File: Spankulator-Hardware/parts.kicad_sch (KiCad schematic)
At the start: 53 parts, among them J10 FRAM Pins, J11 OLED Pins, J14 Eurorack Power Cable, M1 FRAM_Module, M2 OLED, U10 CD4013BE split, U11 TL072CP full, U12 TL072CP full, U7 TL072CP split, U8 TL072CP split, U9 MAX7480 split

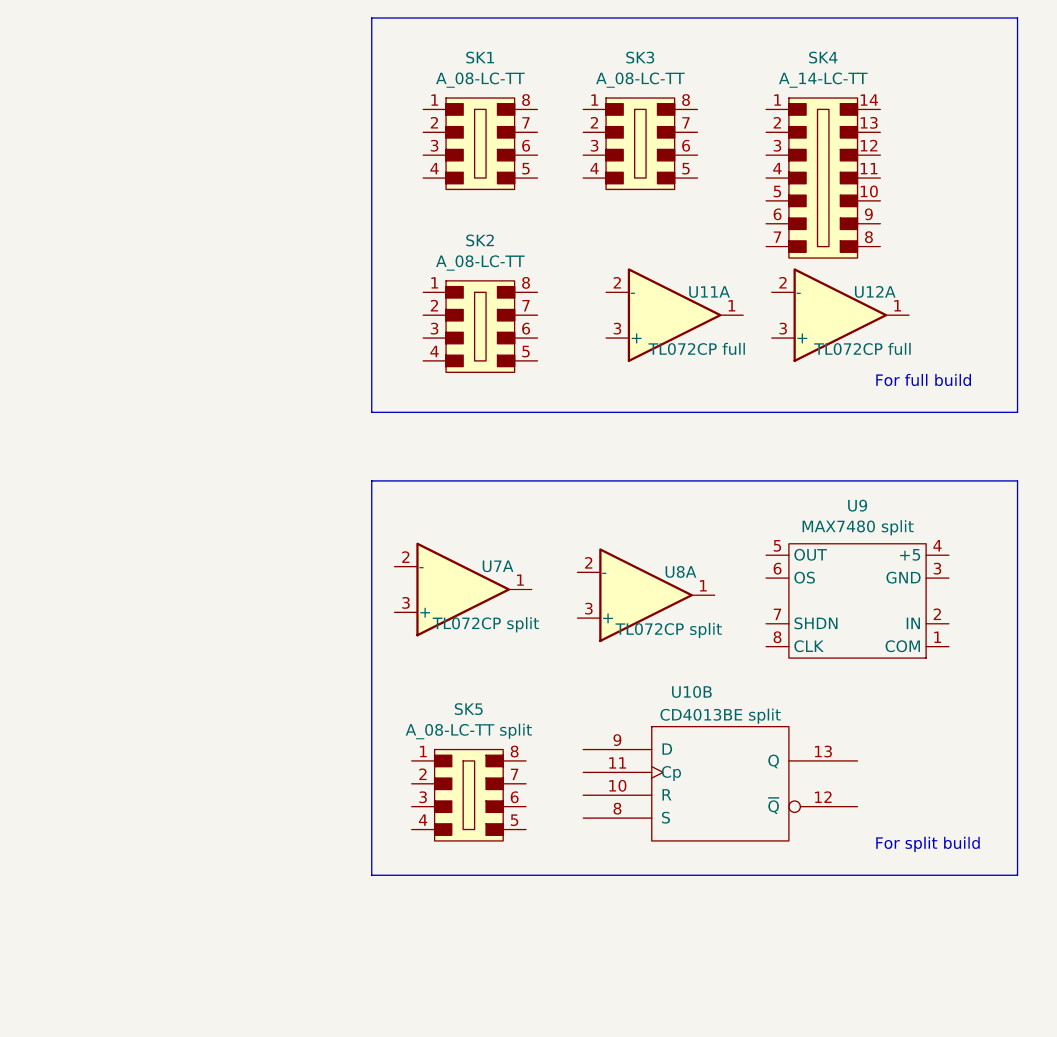
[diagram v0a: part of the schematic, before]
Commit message: v4.4 of Spankulator Board
Many changes to BOM generation. Adds Python scripts.
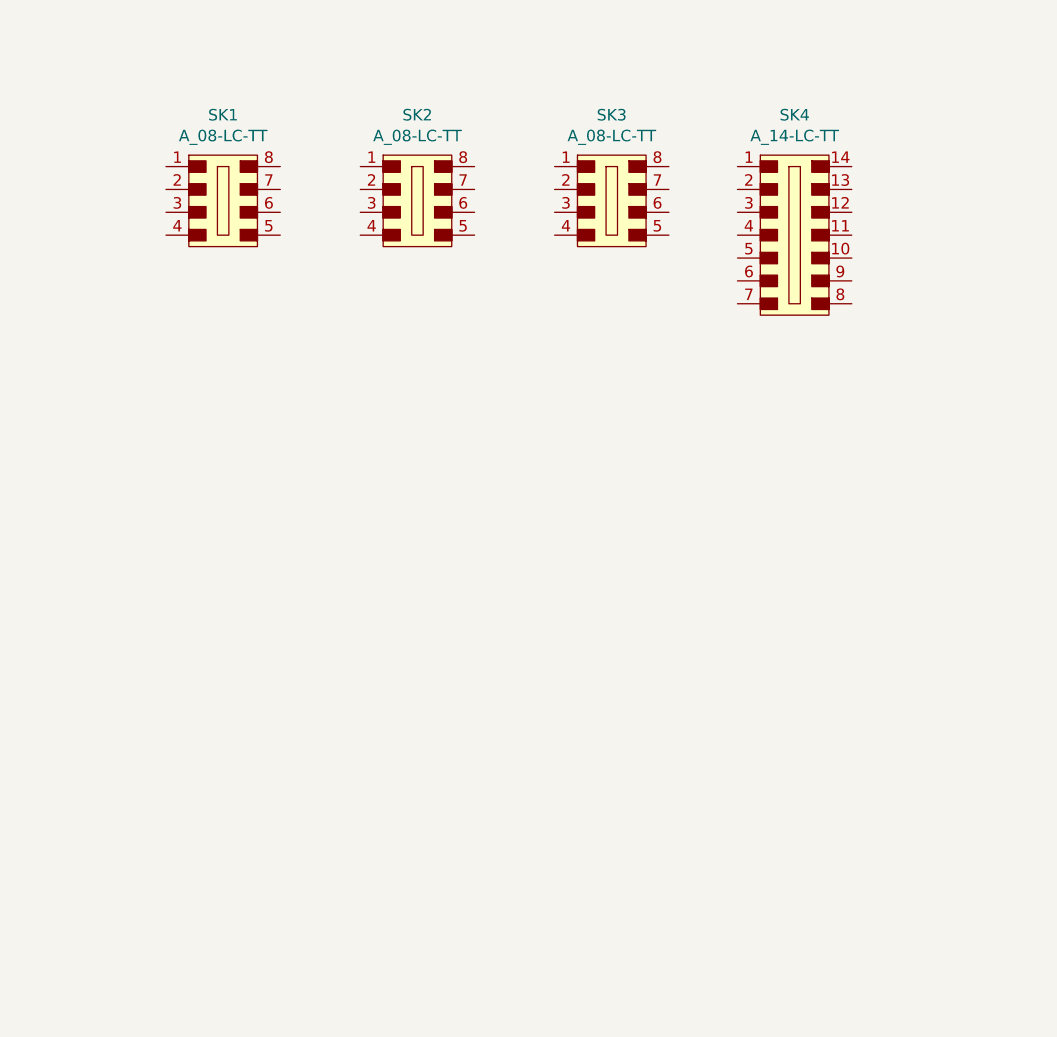
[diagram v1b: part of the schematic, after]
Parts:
- removed SK5: A_08-LC-TT split, Package_DIP:DIP-8_W7.62mm_Socket, symbol dk_Sockets-for-ICs-Transistors:A_08-LC-TT
- removed U10: CD4013BE split, Package_DIP:DIP-14_W7.62mm_Socket, symbol 4xxx_IEEE:4013
- removed U11, U12: TL072CP full, Package_DIP:DIP-8_W7.62mm, symbol Amplifier_Operational:TL072
- removed U7, U8: TL072CP split, Package_DIP:DIP-8_W7.62mm, symbol Amplifier_Operational:TL072
- removed U9: MAX7480 split, Package_DIP:DIP-8_W7.62mm_Socket_LongPads, symbol greenface-symbols:MAX7480
- SK1, SK2, SK3, SK4: Build Type full -> (none)
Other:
- note removed: "For full build"
- note removed: "For split build"
- company: (none) -> Greenface Labs
- title: (none) -> Spankulator
- moved on the sheet: SK1, SK2, SK3, SK4
